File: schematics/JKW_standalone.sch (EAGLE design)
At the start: 225 parts, among them IC1 4093D, IC2 AT-MEGA-328P-AU, IC4 ATMEGA2560-16AU, Q1 BSS84, Q10 BSS84, Q11 BSS84, Q2 BSS84, Q3 BSS84, Q4 BSS84, Q5 BSS84, Q6 BSS84, Q7 BSS84, Q8 BSS84, Q9 BSS84, T1 Mouser: 771-2N7002BK215 , N-C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, T10 Mouser: 771-2N7002BK215 , N-C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, T11 Mouser: 771-2N7002BK215 , N-C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, T12 Mouser: 771-2N7002BK215 , N-C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, T2 Mouser: 771-2N7002BK215 , N-C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, T3 Mouser: 771-2N7002BK215 , N-C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, T4 T-IRLMS6702, T5 Mouser: 771-2N7002BK215 , N-C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, T6 Mouser: 771-2N7002BK215 , N-C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, T7 Mouser: 771-2N7002BK215 , N-C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, T8 Mouser: 771-2N7002BK215 , N-C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, T9 Mouser: 771-2N7002BK215 , N-C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

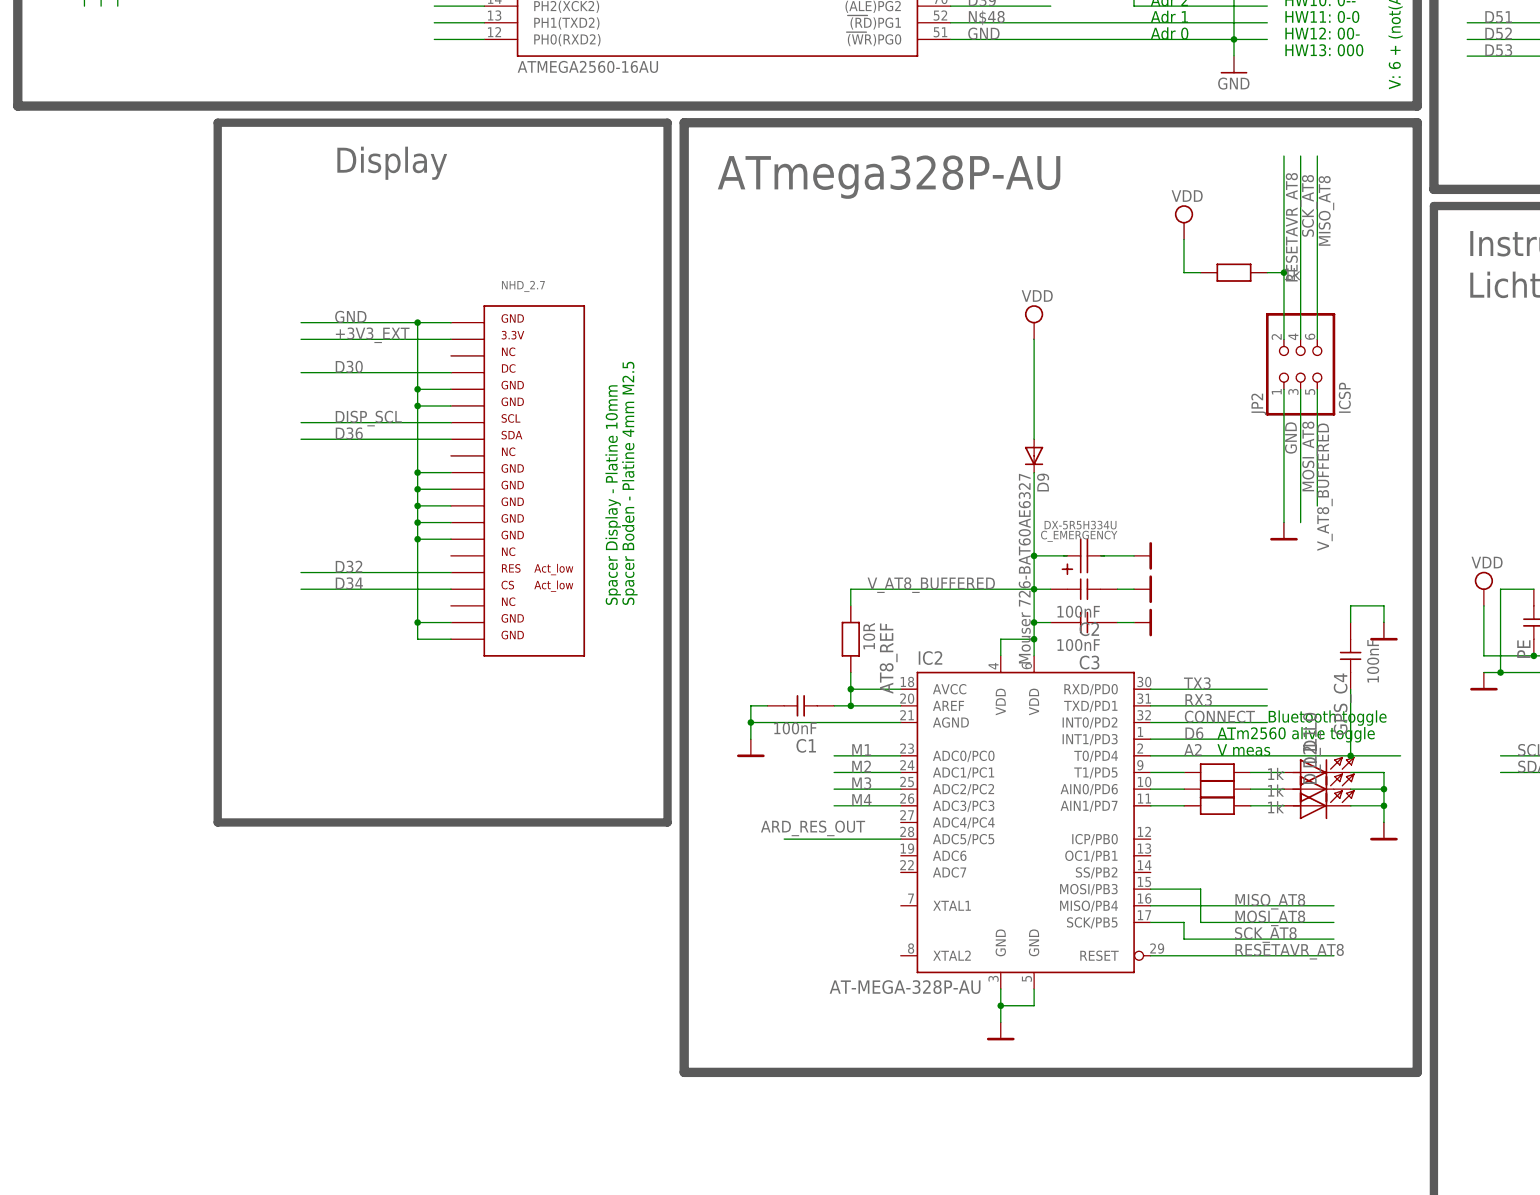
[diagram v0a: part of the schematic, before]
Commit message: changed controller
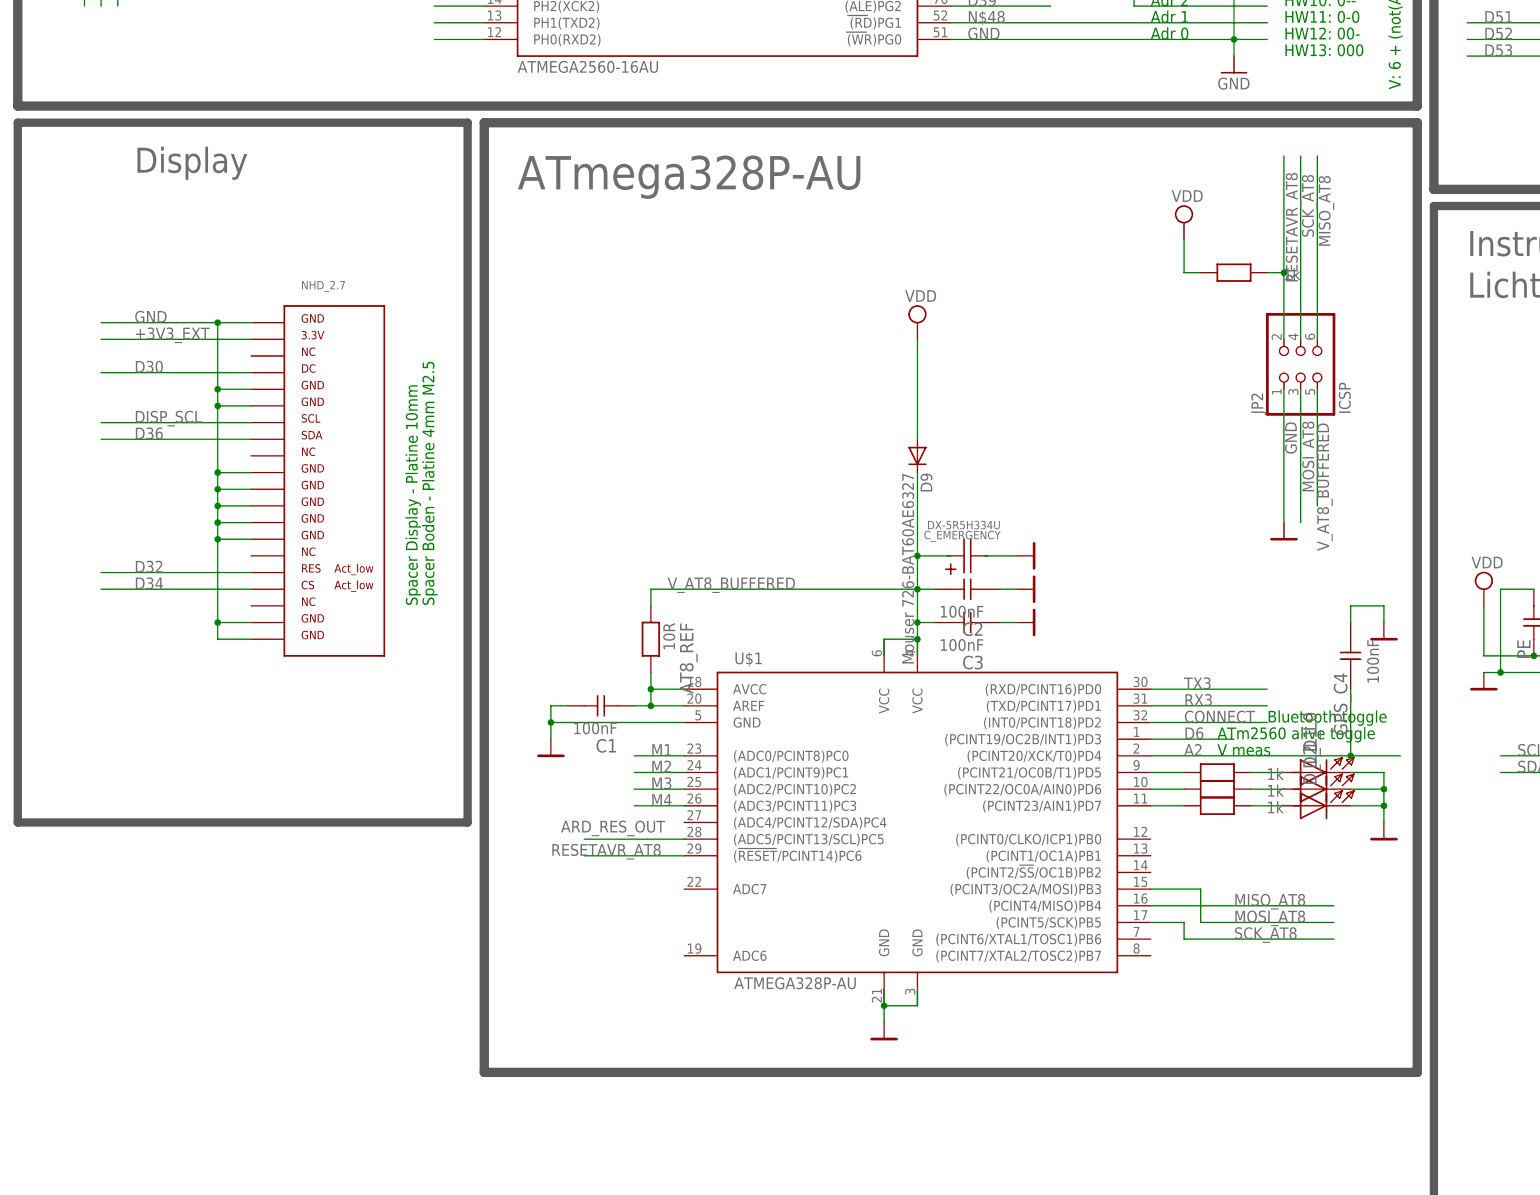
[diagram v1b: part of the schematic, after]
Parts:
- removed IC2: AT-MEGA-328P-AU, µP´s+Pic´s:AT-MEGA-8
- added U$1: ATMEGA328P-AU, Kolja:ATMEGA328P-AU
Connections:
- net A2: now also U$1.(PCINT20/XCK/T0)PD4; no longer IC2.T0/PD4
- net ARD_RES_OUT: now also U$1.(ADC5/PCINT13/SCL)PC5; no longer IC2.ADC5/PC5
- net CONNECT: now also U$1.(INT0/PCINT18)PD2; no longer IC2.INT0/PD2
- net D6: now also U$1.(PCINT19/OC2B/INT1)PD3; no longer IC2.INT1/PD3
- net GND: now also U$1.GND, U$1.GND@1, U$1.GND@2; no longer IC2.AGND, IC2.GND, IC2.GND@1
- net M1: now also U$1.(ADC0/PCINT8)PC0; no longer IC2.ADC0/PC0
- net M2: now also U$1.(ADC1/PCINT9)PC1; no longer IC2.ADC1/PC1
- net M3: now also U$1.(ADC2/PCINT10)PC2; no longer IC2.ADC2/PC2
- net M4: now also U$1.(ADC3/PCINT11)PC3; no longer IC2.ADC3/PC3
- net MISO_AT8: now also U$1.(PCINT4/MISO)PB4; no longer IC2.MISO/PB4
- net MOSI_AT8: now also U$1.(PCINT3/OC2A/MOSI)PB3; no longer IC2.MOSI/PB3
- net N$14: now also U$1.(PCINT23/AIN1)PD7; no longer IC2.AIN1/PD7
- net N$18: now also U$1.(PCINT22/OC0A/AIN0)PD6; no longer IC2.AIN0/PD6
- net N$20: now also U$1.(PCINT21/OC0B/T1)PD5; no longer IC2.T1/PD5
- net N$3: now also U$1.AREF, U$1.AVCC; no longer IC2.AREF, IC2.AVCC
- net RESETAVR_AT8: no longer IC2.RESET
- net RX3: now also U$1.(TXD/PCINT17)PD1; no longer IC2.TXD/PD1
- net SCK_AT8: now also U$1.(PCINT5/SCK)PB5; no longer IC2.SCK/PB5
- net TX3: now also U$1.(RXD/PCINT16)PD0; no longer IC2.RXD/PD0
- net V_AT8_BUFFERED: now also U$1.VCC@1, U$1.VCC@2; no longer IC2.VDD, IC2.VDD@1
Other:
- moved on the sheet: AT8_REF, C1, C2, C3, C_EMERGENCY, D9
